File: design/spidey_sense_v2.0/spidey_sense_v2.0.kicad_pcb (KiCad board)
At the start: 2 copper layers, 46.7 x 51.3 mm, 37 parts, among them J1 Input_Screw_Terminal, J2 Output_Screw_Terminal, J3 Thermocouple_Terminal, J4 Thermocouple_Terminal, J5 Thermocouple_Terminal, J6 Thermocouple_Terminal, U1 LT1025, U2 LTC1983-5, U3 LT1001, U4 LT1001, U5 LT1001, U6 LT1001

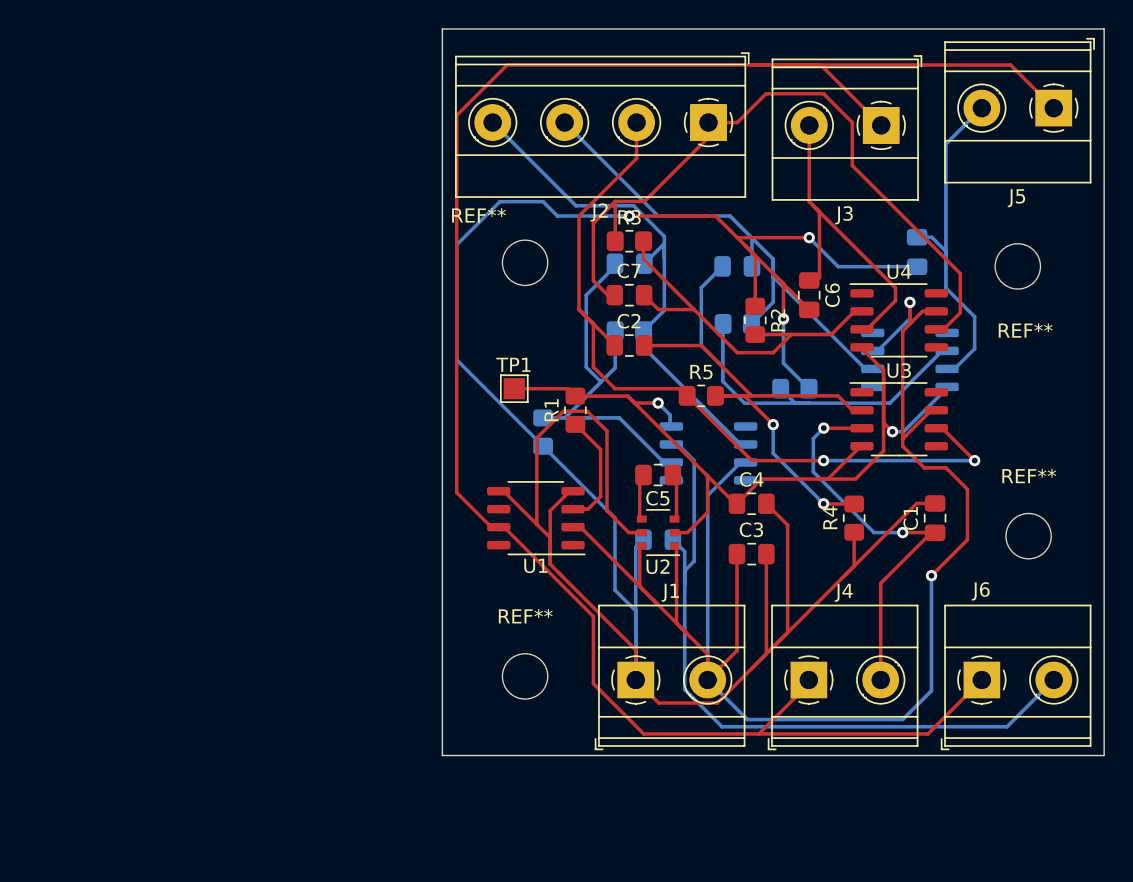
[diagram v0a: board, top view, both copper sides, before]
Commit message: Updated PCB
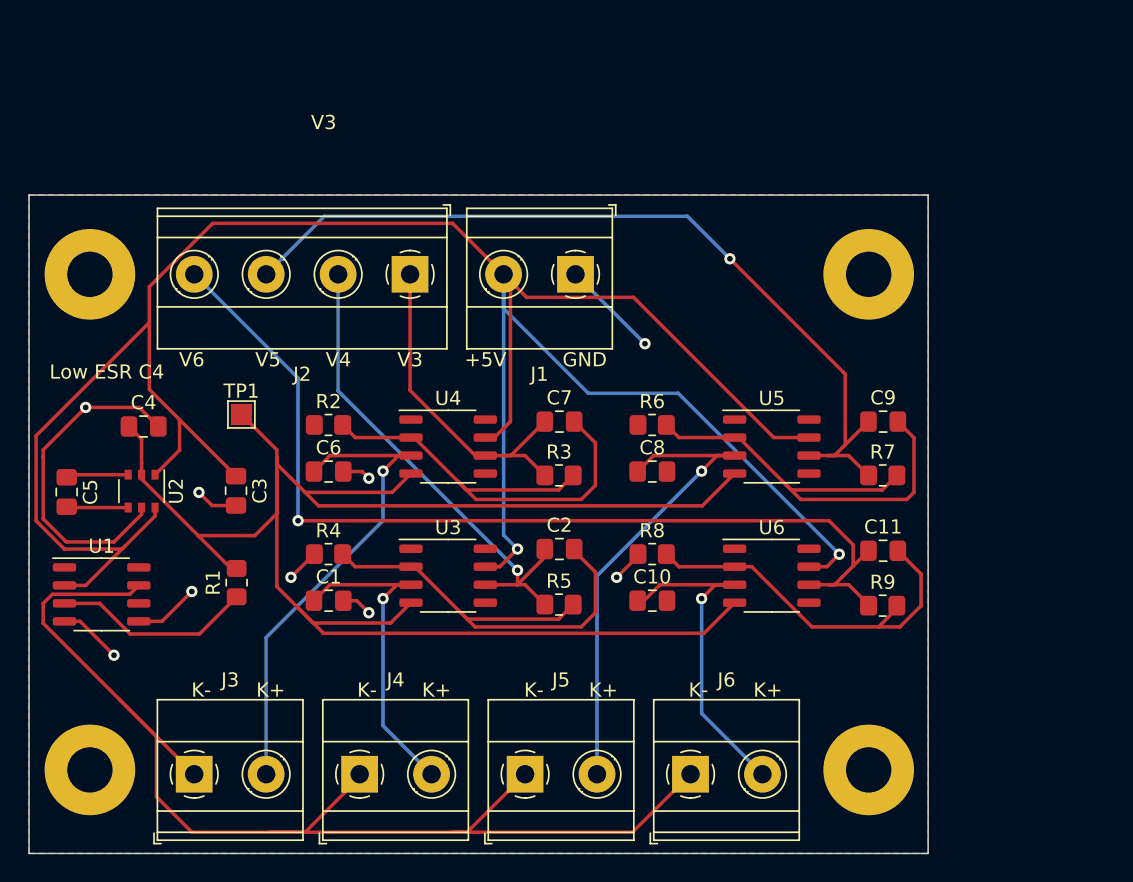
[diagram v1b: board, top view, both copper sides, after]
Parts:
- removed the REF** at (81.5, 65.8)
- removed the REF** at (116.3, 66.0)
- removed the REF** at (117.1, 85.1)
- removed the REF** at (81.5, 95.0)
- added REF**: MountingHole_3.2mm_M3_Pad, MountingHole:MountingHole_3.2mm_M3_Pad, F.Cu at (50.8, 66.6)
- added REF**: MountingHole_3.2mm_M3_Pad, MountingHole:MountingHole_3.2mm_M3_Pad, F.Cu at (105.8, 101.6)
- added REF**: MountingHole_3.2mm_M3_Pad, MountingHole:MountingHole_3.2mm_M3_Pad, F.Cu at (50.8, 101.6)
- added REF**: MountingHole_3.2mm_M3_Pad, MountingHole:MountingHole_3.2mm_M3_Pad, F.Cu at (105.8, 66.6)
- C10, C11, C8, C9, R6, R7, R8, R9, U5, U6: moved to F.Cu
- moved J3 66.7 mm to (58.2, 101.9), turned to 0 degrees
- moved J5 60.1 mm to (81.5, 101.9), turned to 0 degrees
- moved C4 43.3 mm to (54.6, 77.3)
- moved C1 43.2 mm to (67.7, 89.6), turned to 0 degrees
- moved C5 41.8 mm to (49.2, 82.0), turned to -90 degrees
- moved R4 37.2 mm to (67.6, 86.4), turned to 0 degrees
- moved C3 36.7 mm to (61.1, 81.9), turned to -90 degrees
- moved U2 36.6 mm to (54.4, 81.9), turned to -90 degrees
- moved C6 36.2 mm to (67.7, 80.5), turned to 0 degrees
- moved U3 33.7 mm to (76.1, 87.9)
- moved U4 33.1 mm to (76.1, 78.8)
- moved J4 32.4 mm to (69.8, 101.9)
- moved U1 31.1 mm to (51.6, 89.2), turned to 0 degrees
- moved R2 31.0 mm to (67.6, 77.2), turned to 0 degrees
- moved J1 29.0 mm to (85.1, 66.6), turned to 180 degrees
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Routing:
- net GND: track 198.9 -> 51.5 mm, vias 3 -> 9
- net +5V: track 112.3 -> 179.9 mm
- net -5V: track 61.7 -> 122.4 mm, vias 2 -> 0
- net /K-: track 136.2 -> 87.1 mm
- net /Amplifier4/Vout: track 37.0 -> 70.4 mm, vias 0 -> 1
- net /Amplifier1/Vout: track 51.0 -> 24.0 mm
- net /Amplifier4/K+: track 51.0 -> 24.2 mm, vias 0 -> 1
- net /Amplifier3/Vout: track 36.9 -> 60.9 mm, vias 0 -> 1
- net /Amplifier2/Vout: track 56.0 -> 35.3 mm, vias 2 -> 1
- net /Amplifier1/K+: track 23.8 -> 34.6 mm, vias 0 -> 1
- net /Amplifier3/K+: track 24.3 -> 34.6 mm, vias 0 -> 1
- net Net-(C7-Pad2): track 27.1 -> 34.4 mm
- net Net-(R1-Pad1): track 8.06 -> 14.1 mm
- net /Amplifier2/K+: track 28.5 -> 23.5 mm, vias 2 -> 1
- net Net-(C5-Pad1): track 3.22 -> 4.42 mm
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- added copper zone on B.Cu, net GND
- added copper zone on F.Cu, net GND
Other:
- board size 46.7 x 51.3 mm -> 63.5 x 46.5 mm
- board text added: "+5V"
- board text added: "GND"
- board text added: "K+"
- board text added: "K-"
- board text added: "Low ESR C4"
- board text added: "V3"
- board text added: "V4"
- board text added: "V5"
- board text added: "V6"
